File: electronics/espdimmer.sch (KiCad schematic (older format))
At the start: 20 parts, among them J10 LED2, J5 UART, J6 Motion, J7 PWR1, J8 PWR2, J9 LED1, Q1 IRLB3034, Q2 IRLB3034, SW1 Reset, SW2 Flash, U1 ESP-01v090

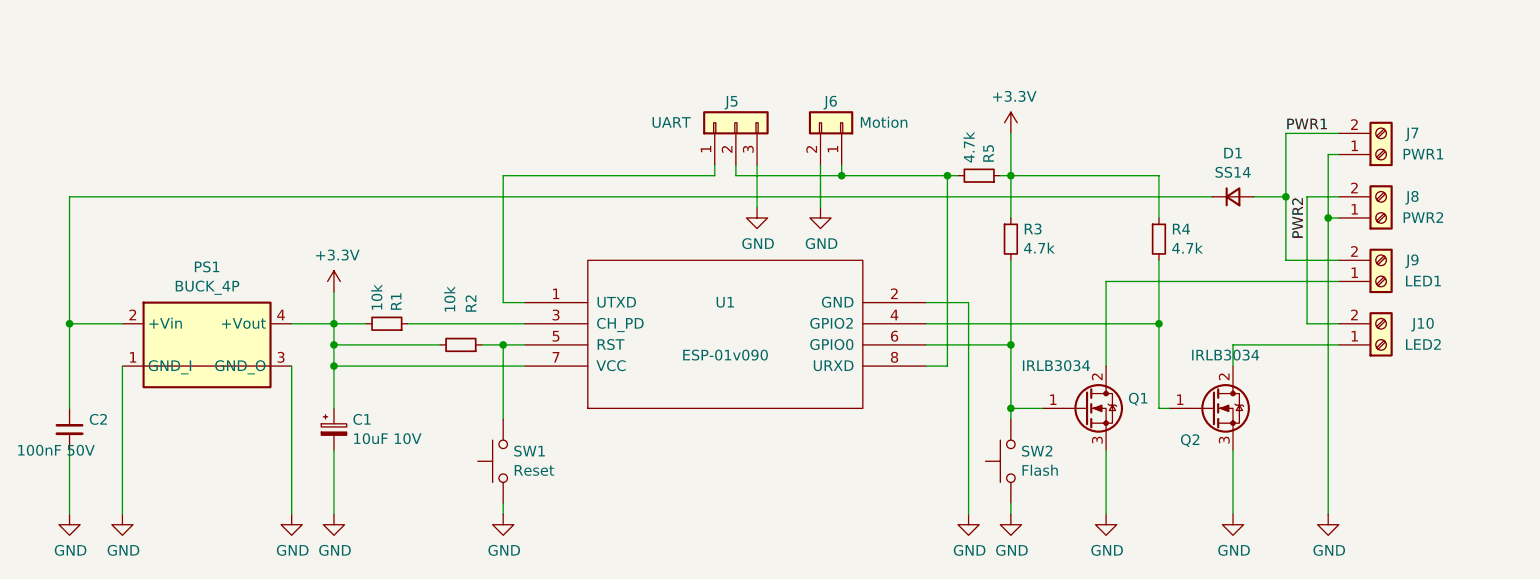
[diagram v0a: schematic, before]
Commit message: Housing added
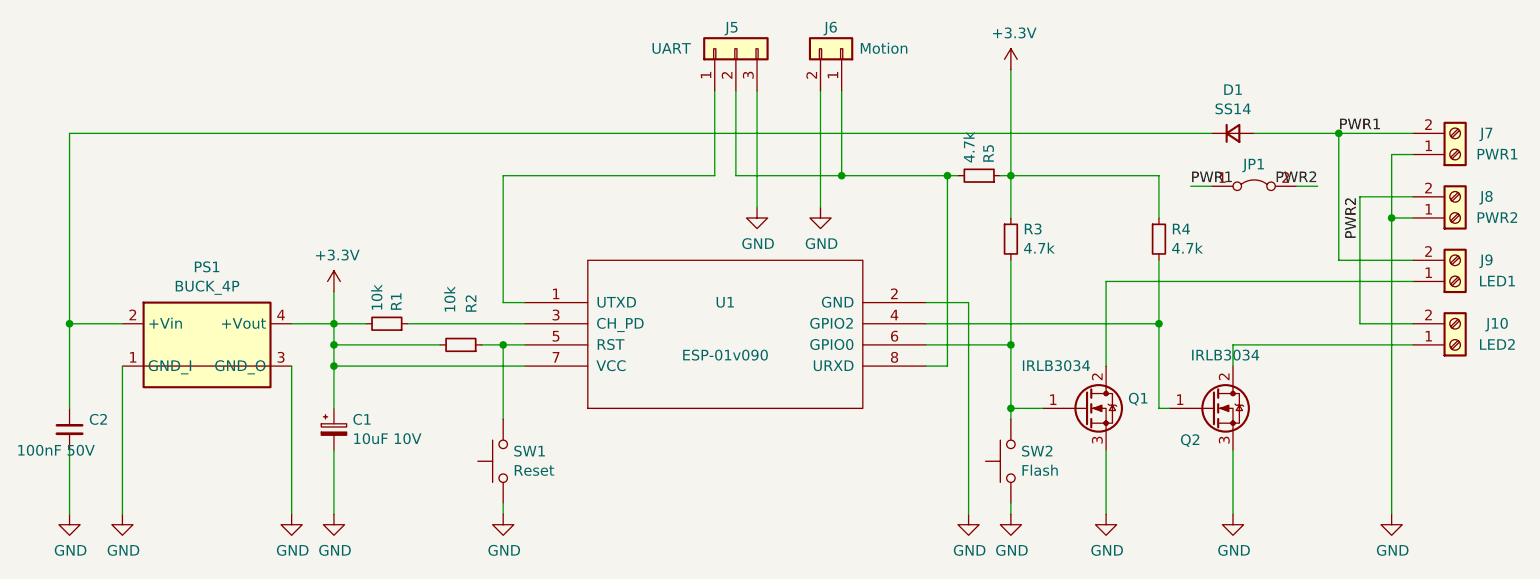
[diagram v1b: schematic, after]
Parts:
- added JP1: Jumper_2_Bridged, Jumper:SolderJumper-2_P1.3mm_Open_TrianglePad1.0x1.5mm, symbol Jumper:Jumper_2_Bridged
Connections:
- net PWR1: now also JP1.1 (A)
- net PWR2: now also JP1.2 (B)
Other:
- moved on the sheet: D1, J10, J5, J6, J7, J8, J9
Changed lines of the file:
@@
 L Connector:Screw_Terminal_01x02 J9
 U 1 1 5FE61684
-P 8700 3450
-F 0 "J9" H 8850 3350 50  0000 C CNN
-F 1 "LED1" H 8900 3450 50  0000 C CNN
-F 2 "TerminalBlock:TerminalBlock_bornier-2_P5.08mm" H 8700 3450 50  0001 C CNN
-F 3 "~" H 8700 3450 50  0001 C CNN
-	1    8700 3450
+P 9050 3450
+F 0 "J9" H 9200 3350 50  0000 C CNN
+F 1 "LED1" H 9250 3450 50  0000 C CNN
+F 2 "TerminalBlock:TerminalBlock_bornier-2_P5.08mm" H 9050 3450 50  0001 C CNN
+F 3 "~" H 9050 3450 50  0001 C CNN
+	1    9050 3450
 	1    0    0    1
 $EndComp
@@
 L Connector:Screw_Terminal_01x02 J10
 U 1 1 5FE62049
-P 8700 3750
-F 0 "J10" H 8900 3650 50  0000 C CNN
-F 1 "LED2" H 8900 3750 50  0000 C CNN
-F 2 "TerminalBlock:TerminalBlock_bornier-2_P5.08mm" H 8700 3750 50  0001 C CNN
-F 3 "~" H 8700 3750 50  0001 C CNN
-	1    8700 3750
+P 9050 3750
+F 0 "J10" H 9250 3650 50  0000 C CNN
+F 1 "LED2" H 9250 3750 50  0000 C CNN
+F 2 "TerminalBlock:TerminalBlock_bornier-2_P5.08mm" H 9050 3750 50  0001 C CNN
+F 3 "~" H 9050 3750 50  0001 C CNN
+	1    9050 3750
 	1    0    0    1
 $EndComp
@@
 L power:+3.3V #PWR010
 U 1 1 5FE69127
-P 6950 2750
-F 0 "#PWR010" H 6950 2600 50  0001 C CNN
-F 1 "+3.3V" H 6965 2923 50  0000 C CNN
-F 2 "" H 6950 2750 50  0001 C CNN
-F 3 "" H 6950 2750 50  0001 C CNN
-	1    6950 2750
-	1    0    0    -1
-$EndComp
-Wire Wire Line
-	6950 2750 6950 2950
+P 6950 2450
+F 0 "#PWR010" H 6950 2300 50  0001 C CNN
+F 1 "+3.3V" H 6965 2623 50  0000 C CNN
+F 2 "" H 6950 2450 50  0001 C CNN
+F 3 "" H 6950 2450 50  0001 C CNN
+	1    6950 2450
+	1    0    0    -1
+$EndComp
+Wire Wire Line
+	6950 2450 6950 2950
 Connection ~ 6950 2950
 Wire Wire Line
@@
 Connection ~ 6950 4050
 Wire Wire Line
-	8500 3450 7400 3450
-Wire Wire Line
 	7400 3450 7400 3850
 Wire Wire Line
-	5750 3100 5750 2900
+	5750 3100 5750 2550
 Wire Wire Line
 	6650 2950 6150 2950
 Wire Wire Line
-	5650 2950 5650 2900
+	5650 2950 5650 2550
 Wire Wire Line
 	4550 2950 5550 2950
 Wire Wire Line
-	5550 2950 5550 2900
+	5550 2950 5550 2550
 $Comp
 L Connector_Generic:Conn_01x02 J6
 U 1 1 5FEBA2DD
-P 6150 2700
-F 0 "J6" V 6250 2650 50  0000 C CNN
-F 1 "Motion" V 6150 2900 50  0000 C CNN
-F 2 "Connector_PinHeader_2.54mm:PinHeader_1x02_P2.54mm_Vertical" H 6150 2700 50  0001 C CNN
-F 3 "~" H 6150 2700 50  0001 C CNN
-	1    6150 2700
+P 6150 2350
+F 0 "J6" V 6250 2300 50  0000 C CNN
+F 1 "Motion" V 6150 2550 50  0000 C CNN
+F 2 "Connector_PinHeader_2.54mm:PinHeader_1x02_P2.54mm_Vertical" H 6150 2350 50  0001 C CNN
+F 3 "~" H 6150 2350 50  0001 C CNN
+	1    6150 2350
 	0    1    -1   0
 $EndComp
@@
 	8000 4250 8000 4550
 Wire Wire Line
-	8500 3150 8450 3150
-Wire Wire Line
-	8450 3150 8450 4550
-Wire Wire Line
-	8450 3150 8450 2850
-Wire Wire Line
-	8450 2850 8500 2850
-Connection ~ 8450 3150
-Wire Wire Line
-	8500 3650 8350 3650
-Wire Wire Line
-	8350 3650 8350 3050
-Wire Wire Line
-	8350 3050 8500 3050
-Wire Wire Line
-	8500 3350 8250 3350
-Wire Wire Line
-	8250 2750 8500 2750
-Wire Wire Line
-	6150 2900 6150 2950
+	8850 3150 8750 3150
+Wire Wire Line
+	8750 3150 8750 4550
+Wire Wire Line
+	8750 3150 8750 2850
+Wire Wire Line
+	8750 2850 8850 2850
+Connection ~ 8750 3150
+Wire Wire Line
+	8850 3650 8600 3650
+Wire Wire Line
+	8600 3050 8850 3050
+Wire Wire Line
+	8850 3350 8500 3350
+Wire Wire Line
+	8500 2750 8850 2750
+Wire Wire Line
+	6150 2550 6150 2950
 Connection ~ 6150 2950
 Wire Wire Line
 	6150 2950 5650 2950
 Wire Wire Line
-	6050 2900 6050 3100
+	6050 2550 6050 3100
 $Comp
 L power:GND #PWR08
@@
 L Connector_Generic:Conn_01x03 J5
 U 1 1 5FE252C1
-P 5650 2700
-F 0 "J5" V 5750 2750 50  0000 R CNN
-F 1 "UART" V 5650 3100 50  0000 R CNN
-F 2 "Connector_PinHeader_2.54mm:PinHeader_1x03_P2.54mm_Vertical" H 5650 2700 50  0001 C CNN
-F 3 "~" H 5650 2700 50  0001 C CNN
-	1    5650 2700
+P 5650 2350
+F 0 "J5" V 5750 2400 50  0000 R CNN
+F 1 "UART" V 5650 2750 50  0000 R CNN
+F 2 "Connector_PinHeader_2.54mm:PinHeader_1x03_P2.54mm_Vertical" H 5650 2350 50  0001 C CNN
+F 3 "~" H 5650 2350 50  0001 C CNN
+	1    5650 2350
 	0    -1   -1   0
 $EndComp
@@
 L Connector:Screw_Terminal_01x02 J7
 U 1 1 5FF5CAAF
-P 8700 2850
-F 0 "J7" H 8850 2750 50  0000 C CNN
-F 1 "PWR1" H 8900 2850 50  0000 C CNN
-F 2 "TerminalBlock:TerminalBlock_bornier-2_P5.08mm" H 8700 2850 50  0001 C CNN
-F 3 "~" H 8700 2850 50  0001 C CNN
-	1    8700 2850
+P 9050 2850
+F 0 "J7" H 9200 2750 50  0000 C CNN
+F 1 "PWR1" H 9250 2850 50  0000 C CNN
+F 2 "TerminalBlock:TerminalBlock_bornier-2_P5.08mm" H 9050 2850 50  0001 C CNN
+F 3 "~" H 9050 2850 50  0001 C CNN
+	1    9050 2850
 	1    0    0    1
 $EndComp
 Wire Wire Line
-	2500 3050 2500 3650
-Wire Wire Line
-	2500 3050 7900 3050
-Wire Wire Line
-	8250 3350 8250 3050
-Connection ~ 8250 3050
-Wire Wire Line
-	8250 3050 8250 2750
+	2500 2750 2500 3650
+Wire Wire Line
+	2500 2750 7900 2750
+Wire Wire Line
+	8500 3350 8500 2750
+Connection ~ 8500 2750
 $Comp
 L Device:CP_Small C1
@@
 $EndComp
 Wire Wire Line
-	8500 3750 8000 3750
+	8850 3750 8000 3750
 Wire Wire Line
 	8000 3750 8000 3850
@@
 L Connector:Screw_Terminal_01x02 J8
 U 1 1 5FE24A4C
-P 8700 3150
-F 0 "J8" H 8850 3050 50  0000 C CNN
-F 1 "PWR2" H 8900 3150 50  0000 C CNN
-F 2 "TerminalBlock:TerminalBlock_bornier-2_P5.08mm" H 8700 3150 50  0001 C CNN
-F 3 "~" H 8700 3150 50  0001 C CNN
-	1    8700 3150
+P 9050 3150
+F 0 "J8" H 9200 3050 50  0000 C CNN
+F 1 "PWR2" H 9250 3150 50  0000 C CNN
+F 2 "TerminalBlock:TerminalBlock_bornier-2_P5.08mm" H 9050 3150 50  0001 C CNN
+F 3 "~" H 9050 3150 50  0001 C CNN
+	1    9050 3150
 	1    0    0    1
 $EndComp
@@
 Wire Wire Line
 	7400 4250 7400 4550
-Text Label 8250 2750 0    50   ~ 0
+Text Label 8500 2750 0    50   ~ 0
 PWR1
-Text Label 8350 3050 3    50   ~ 0
-PWR2
 $Comp
 L Device:R_Small R5
@@
 L Device:D_Small D1
 U 1 1 600C3ECC
-P 8000 3050
-F 0 "D1" H 8000 3255 50  0000 C CNN
-F 1 "SS14" H 8000 3164 50  0000 C CNN
-F 2 "Diode_SMD:D_SMA_Handsoldering" V 8000 3050 50  0001 C CNN
-F 3 "~" V 8000 3050 50  0001 C CNN
-	1    8000 3050
-	1    0    0    -1
-$EndComp
-Wire Wire Line
-	8100 3050 8250 3050
+P 8000 2750
+F 0 "D1" H 8000 2955 50  0000 C CNN
+F 1 "SS14" H 8000 2864 50  0000 C CNN
+F 2 "Diode_SMD:D_SMA_Handsoldering" V 8000 2750 50  0001 C CNN
+F 3 "~" V 8000 2750 50  0001 C CNN
+	1    8000 2750
+	1    0    0    -1
+$EndComp
+Wire Wire Line
+	8100 2750 8500 2750
 Wire Wire Line
 	2500 4050 2500 3650
@@
 L power:GND #PWR0105
 U 1 1 600FD215
-P 8450 4550
-F 0 "#PWR0105" H 8450 4300 50  0001 C CNN
-F 1 "GND" H 8455 4377 50  0000 C CNN
-F 2 "" H 8450 4550 50  0001 C CNN
-F 3 "" H 8450 4550 50  0001 C CNN
-	1    8450 4550
+P 8750 4550
+F 0 "#PWR0105" H 8750 4300 50  0001 C CNN
+F 1 "GND" H 8755 4377 50  0000 C CNN
+F 2 "" H 8750 4550 50  0001 C CNN
+F 3 "" H 8750 4550 50  0001 C CNN
+	1    8750 4550
 	1    0    0    -1
 $EndComp
@@
 	1    0    0    -1
 $EndComp
+$Comp
+L Jumper:Jumper_2_Bridged JP1
+U 1 1 60A05F3F
+P 8100 3000
+F 0 "JP1" H 8100 3103 50  0000 C CNN
+F 1 "Jumper_2_Bridged" H 8100 3104 50  0001 C CNN
+F 2 "Jumper:SolderJumper-2_P1.3mm_Open_TrianglePad1.0x1.5mm" H 8100 3000 50  0001 C CNN
+F 3 "~" H 8100 3000 50  0001 C CNN
+	1    8100 3000
+	1    0    0    -1
+$EndComp
+Wire Wire Line
+	8600 3050 8600 3650
+Text Label 8600 3050 3    50   ~ 0
+PWR2
+Wire Wire Line
+	7400 3450 8850 3450
+Wire Wire Line
+	7800 3000 7900 3000
+Wire Wire Line
+	8400 3000 8300 3000
+Text Label 7800 3000 0    50   ~ 0
+PWR1
+Text Label 8400 3000 2    50   ~ 0
+PWR2
 $EndSCHEMATC
